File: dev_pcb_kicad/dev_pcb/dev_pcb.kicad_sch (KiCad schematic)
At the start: 1 part, among them U1 XIAO-ESP32-S3-SMD

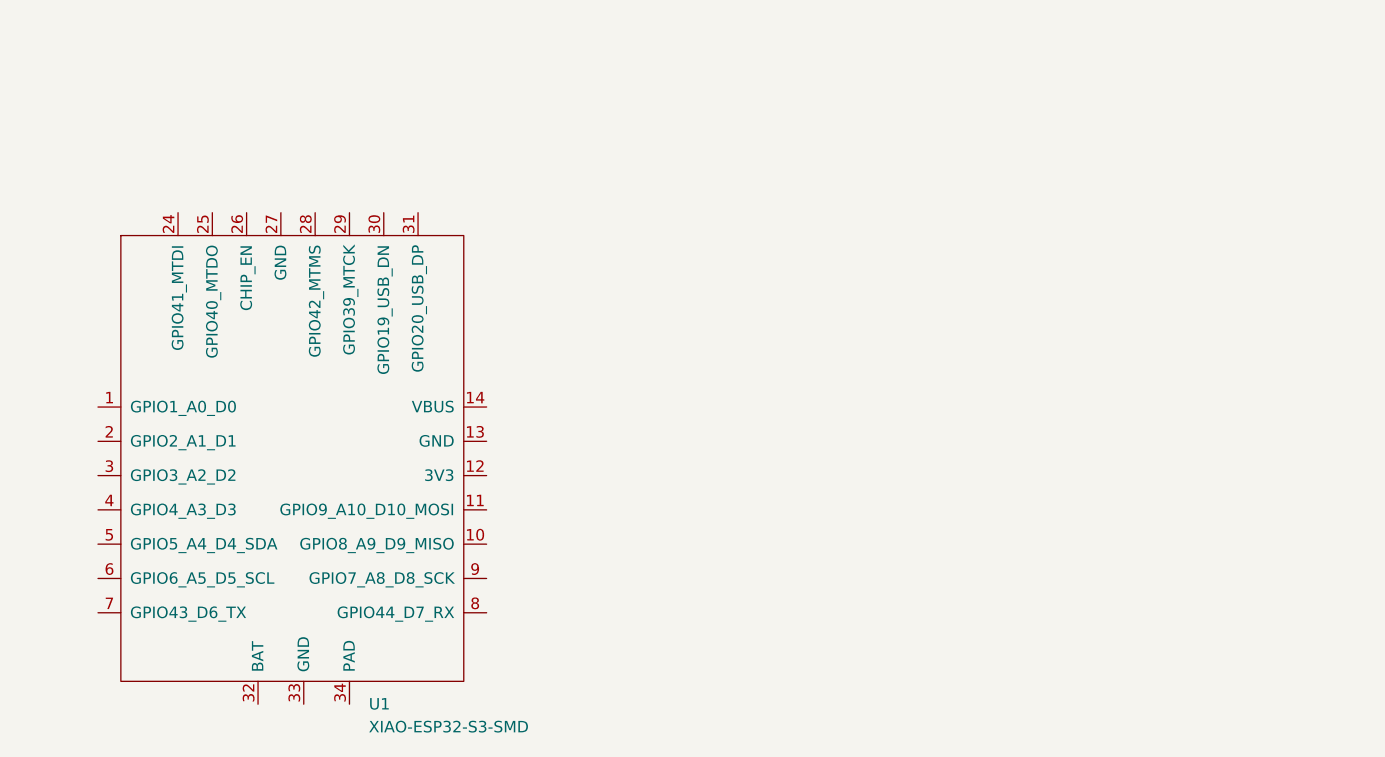
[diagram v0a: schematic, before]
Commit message: mk1 pcb
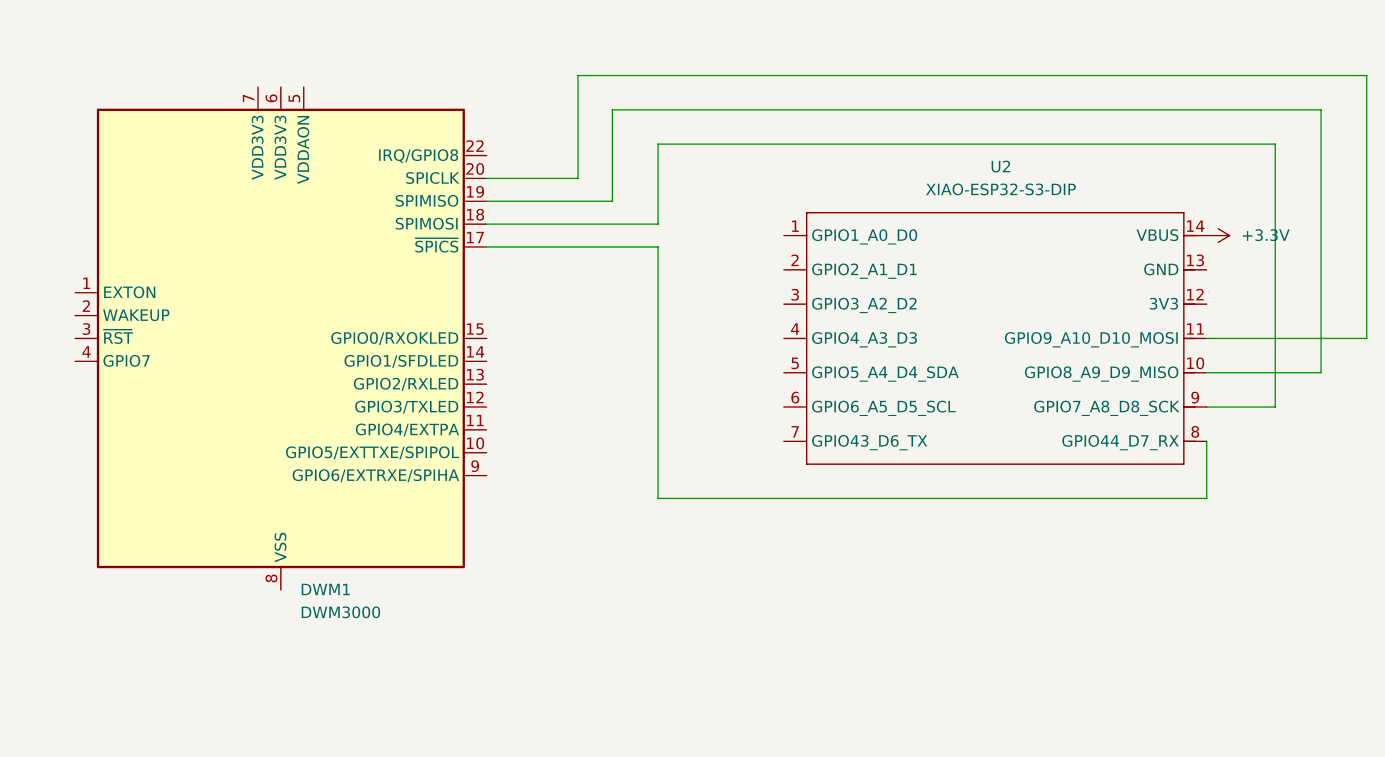
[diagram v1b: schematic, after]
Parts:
- removed U1: XIAO-ESP32-S3-SMD, XIAO_Series_Footprints:XIAO-ESP32-S3-SMD, symbol Seeed_Studio_XIAO_Series:XIAO-ESP32-S3-SMD
- added DWM1: DWM3000, RF_Module:DWM1000, symbol RF_Module:DWM3000
- added U2: XIAO-ESP32-S3-DIP, XIAO_Series_Footprints:XIAO-ESP32-S3-DIP, symbol Seeed_Studio_XIAO_Series:XIAO-ESP32-S3-DIP
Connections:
- new net: DWM1.16 (VSS), DWM1.21 (VSS), DWM1.23 (VSS), DWM1.24 (VSS), DWM1.8 (VSS)
- new net: DWM1.17 (~{SPICS}), U2.8 (GPIO44_D7_RX)
- new net: DWM1.18 (SPIMOSI), U2.9 (GPIO7_A8_D8_SCK)
- new net: DWM1.19 (SPIMISO), U2.10 (GPIO8_A9_D9_MISO)
- new net: DWM1.20 (SPICLK), U2.11 (GPIO9_A10_D10_MOSI)
- new net +3.3V: U2.14 (VBUS)

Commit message: .
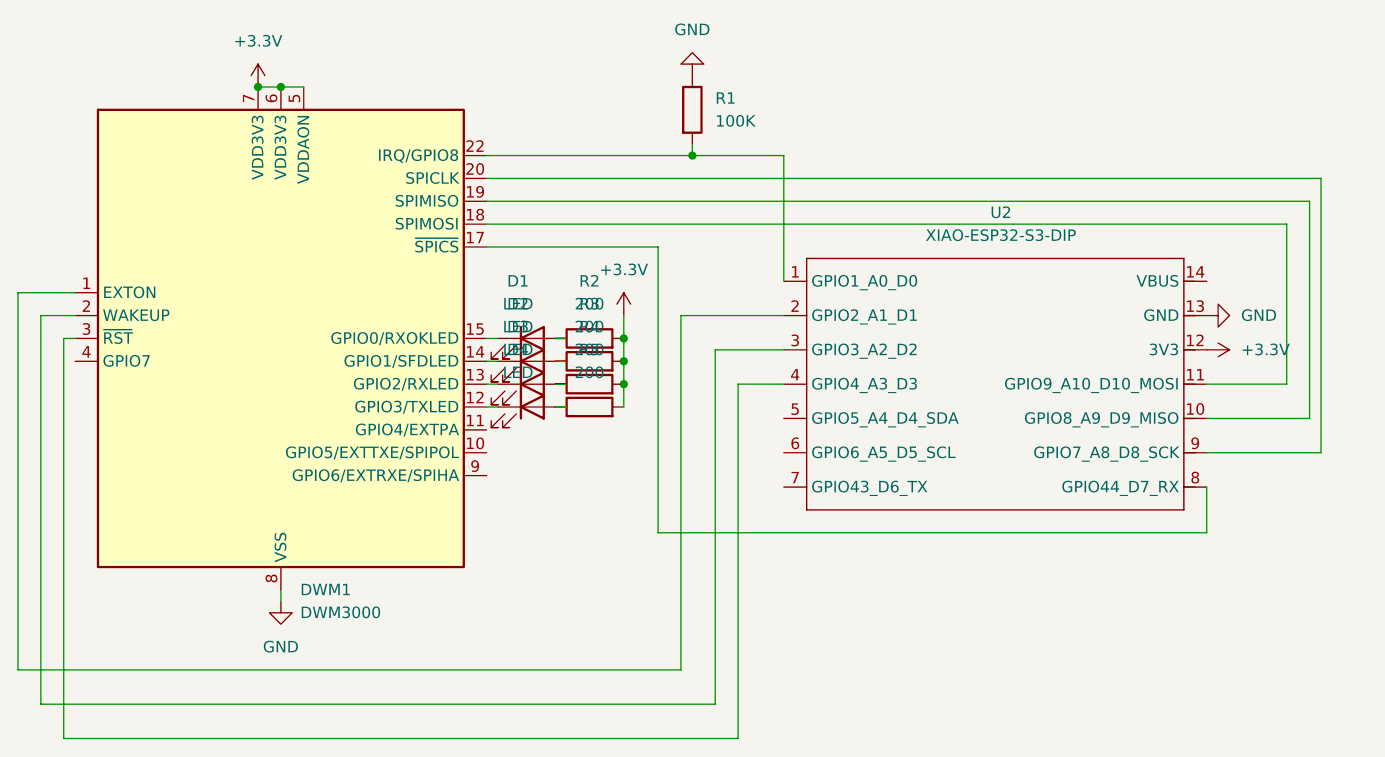
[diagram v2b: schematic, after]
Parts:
- added D1, D2, D3, D4: LED, LED_SMD:LED_0402_1005Metric_Pad0.77x0.64mm_HandSolder, symbol Device:LED
- added R1: 100K, Resistor_SMD:R_0603_1608Metric_Pad0.98x0.95mm_HandSolder, symbol Device:R
- added R2, R3, R4, R5: 200, Resistor_SMD:R_0805_2012Metric_Pad1.20x1.40mm_HandSolder, symbol Device:R
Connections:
- net +3.3V: now also DWM1.5 (VDDAON), DWM1.6 (VDD3V3), DWM1.7 (VDD3V3), U2.12 (3V3), R2.2, R3.2, R4.2, R5.2; no longer U2.14 (VBUS)
- net at DWM1.1 (EXTON): now also U2.2 (GPIO2_A1_D1)
- net at DWM1.12 (GPIO3/TXLED): now also D4.1 (K)
- net at DWM1.13 (GPIO2/RXLED): now also D3.1 (K)
- net at DWM1.14 (GPIO1/SFDLED): now also D2.1 (K)
- net at DWM1.15 (GPIO0/RXOKLED): now also D1.1 (K)
- net GND: now reaches DWM1.16 (VSS), DWM1.21 (VSS), DWM1.23 (VSS), DWM1.24 (VSS), DWM1.8 (VSS)
- net GND: now also U2.13 (GND), R1.1
- net at DWM1.18 (SPIMOSI): now also U2.11 (GPIO9_A10_D10_MOSI); no longer U2.9 (GPIO7_A8_D8_SCK)
- net at DWM1.2 (WAKEUP): now also U2.3 (GPIO3_A2_D2)
- net at DWM1.20 (SPICLK): now also U2.9 (GPIO7_A8_D8_SCK); no longer U2.11 (GPIO9_A10_D10_MOSI)
- net at DWM1.22 (IRQ/GPIO8): now also U2.1 (GPIO1_A0_D0), R1.2
- net at DWM1.3 (~{RST}): now also U2.4 (GPIO4_A3_D3)
- new net: D1.2 (A), R2.1
- new net: D4.2 (A), R5.1
- new net: D2.2 (A), R3.1
- new net: D3.2 (A), R4.1
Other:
- moved on the sheet: U2
